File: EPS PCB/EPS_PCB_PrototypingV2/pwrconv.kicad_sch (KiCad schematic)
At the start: 35 parts, among them J3 Conn_01x02_Pin, J4 Conn_01x02_Pin, J5 Conn_01x02_Pin, J6 Conn_01x02_Pin, U1 TPS5430DDA, U2 TPS5430DDA, U3 TPS5430DDA, U4 TPS7A1650DGNR

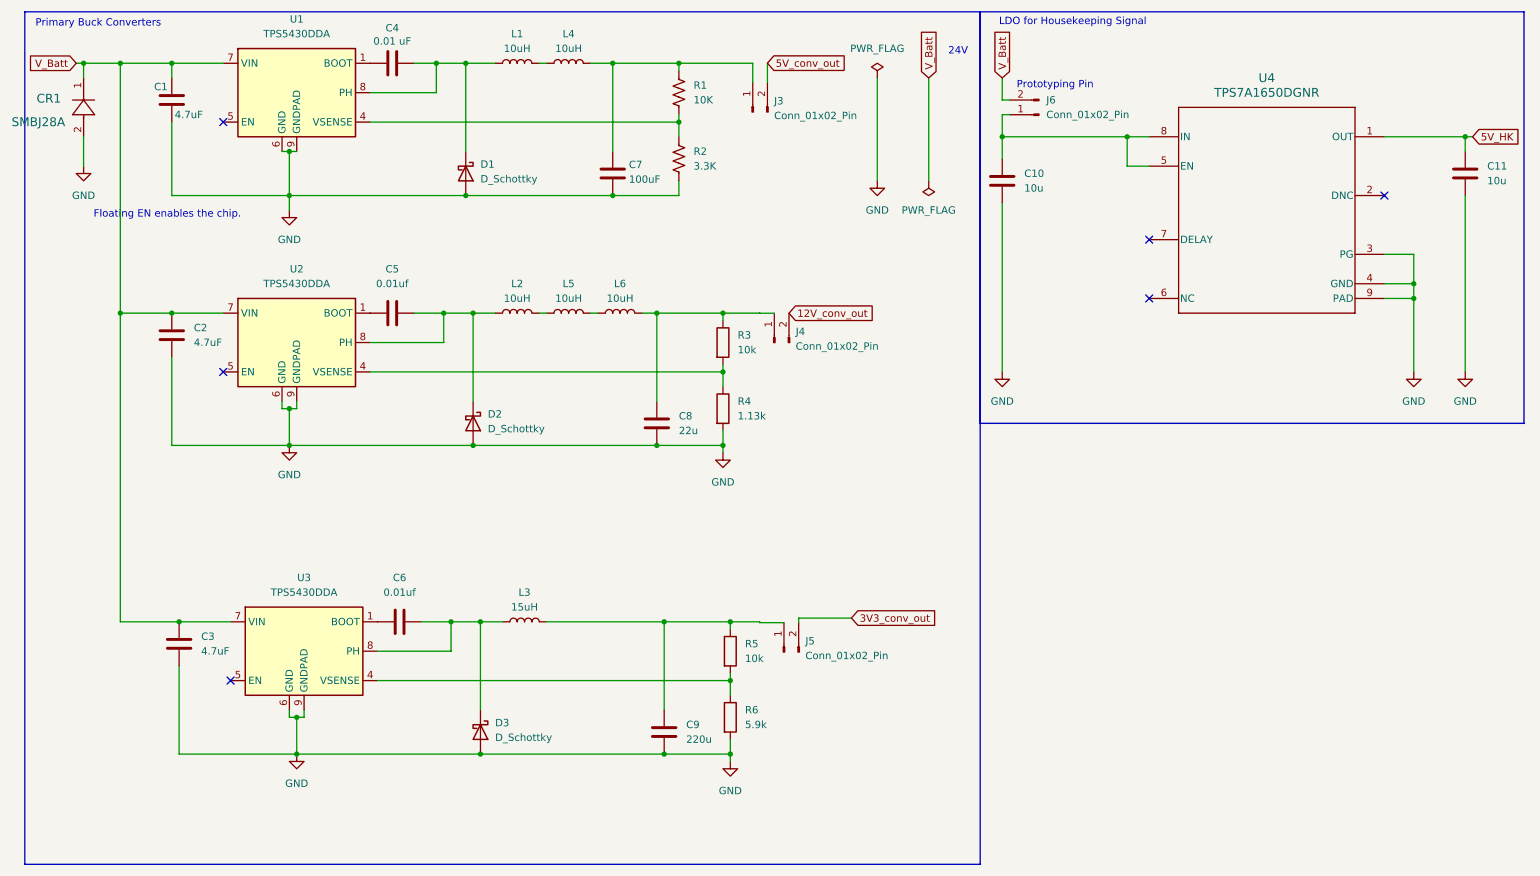
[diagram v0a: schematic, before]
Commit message: EPS PCB Ready for Order
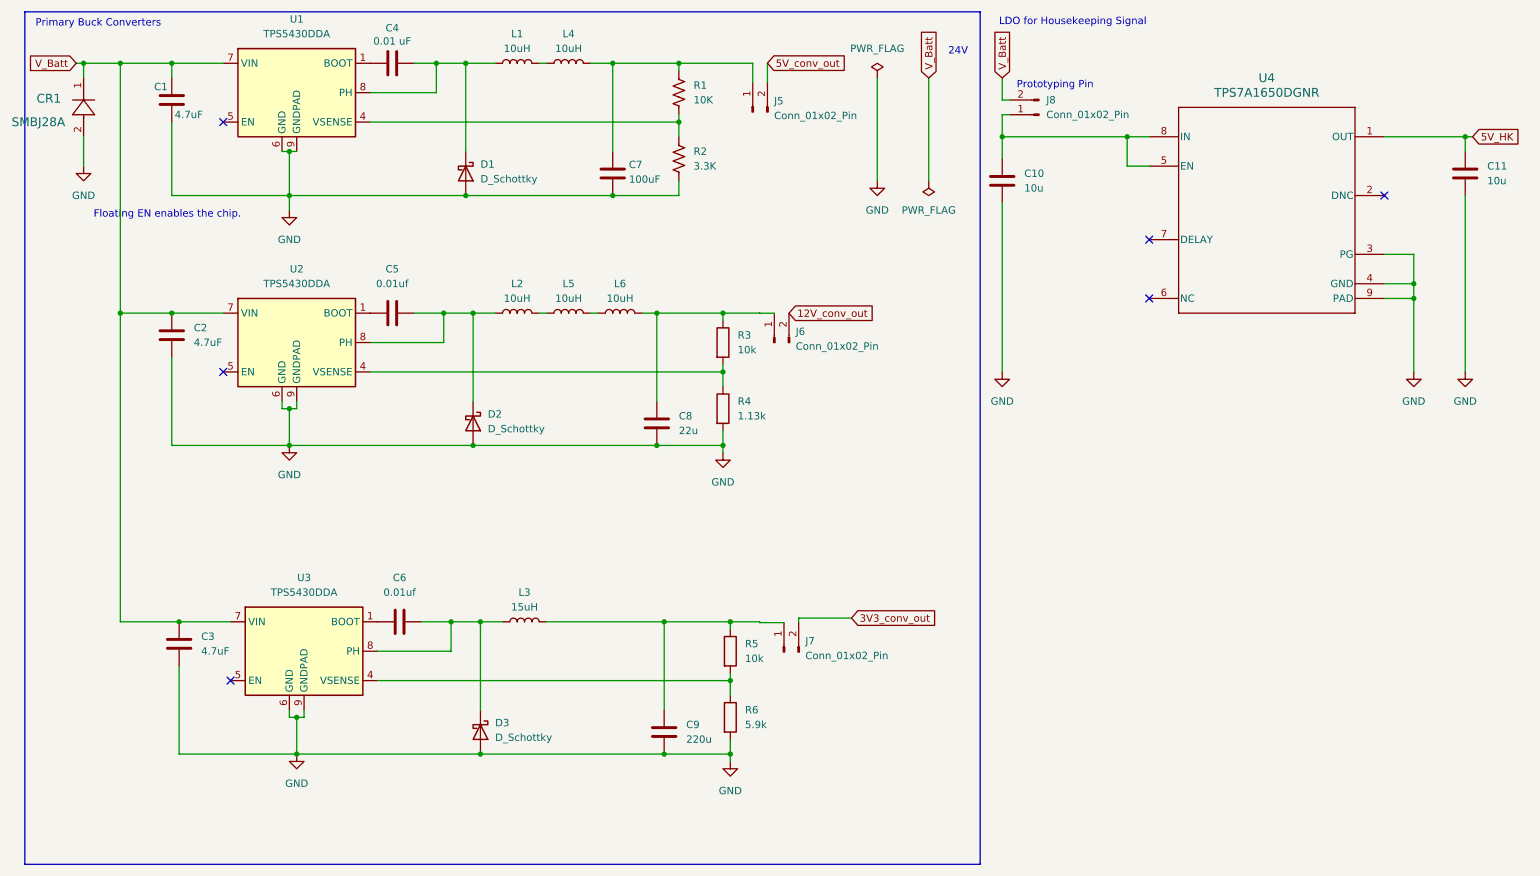
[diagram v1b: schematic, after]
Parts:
- renumbered J3 to J5, J4 to J6, J5 to J7, J6 to J8
